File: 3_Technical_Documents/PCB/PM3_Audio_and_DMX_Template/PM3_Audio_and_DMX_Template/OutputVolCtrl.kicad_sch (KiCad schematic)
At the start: 1 part

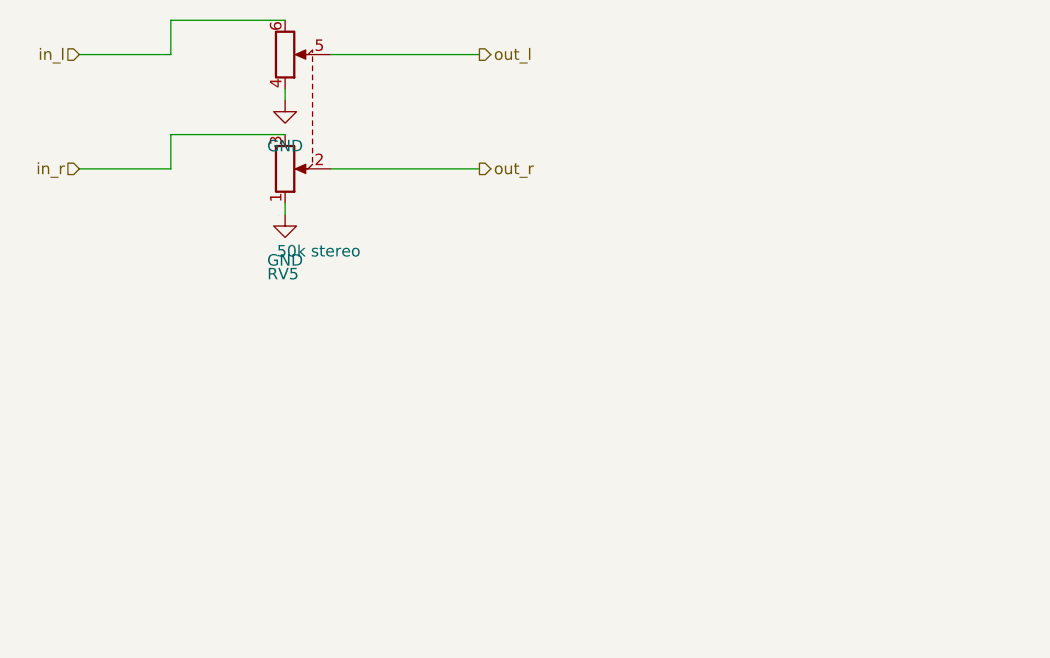
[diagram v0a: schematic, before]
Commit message: new push
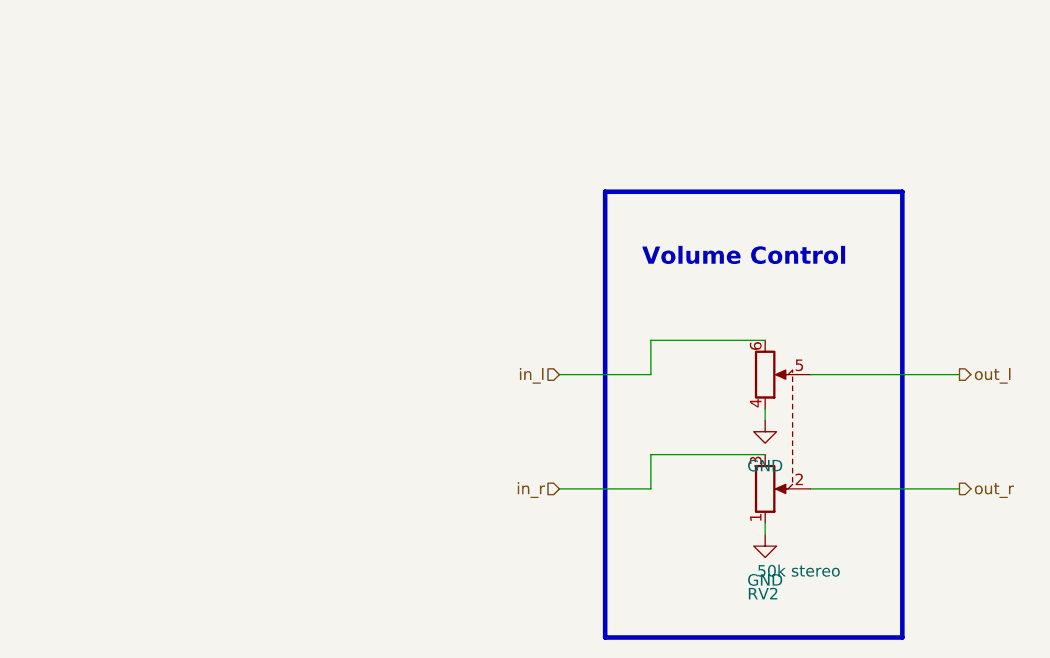
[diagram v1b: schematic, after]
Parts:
- renumbered RV5 to RV2
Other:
- note added: "Volume Control"
- moved on the sheet: RV2
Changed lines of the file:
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@@
 	(generator_version "9.0")
 	(paper "A4")
-	(wire
-		(pts
-			(xy 148.59 88.9) (xy 158.75 88.9)
-		)
-		(stroke
-			(width 0)
-			(type default)
-		)
-	)
-	(wire
-		(pts
-			(xy 158.75 85.09) (xy 171.45 85.09)
-		)
-		(stroke
-			(width 0)
-			(type default)
-		)
-	)
-	(wire
-		(pts
-			(xy 158.75 101.6) (xy 158.75 97.79)
-		)
-		(stroke
-			(width 0)
-			(type default)
-		)
-	)
-	(wire
-		(pts
-			(xy 171.45 105.41) (xy 171.45 106.68)
-		)
-		(stroke
-			(width 0)
-			(type default)
-		)
-	)
-	(wire
-		(pts
-			(xy 158.75 97.79) (xy 171.45 97.79)
-		)
-		(stroke
-			(width 0)
-			(type default)
-		)
-	)
-	(wire
-		(pts
-			(xy 176.53 88.9) (xy 193.04 88.9)
-		)
-		(stroke
-			(width 0)
-			(type default)
-		)
-	)
-	(wire
-		(pts
-			(xy 148.59 101.6) (xy 158.75 101.6)
-		)
-		(stroke
-			(width 0)
-			(type default)
-		)
-	)
-	(wire
-		(pts
-			(xy 176.53 101.6) (xy 193.04 101.6)
-		)
-		(stroke
-			(width 0)
-			(type default)
-		)
-	)
-	(wire
-		(pts
-			(xy 158.75 88.9) (xy 158.75 85.09)
-		)
-		(stroke
-			(width 0)
-			(type default)
-		)
-	)
-	(wire
-		(pts
-			(xy 171.45 92.71) (xy 171.45 93.98)
+	(rectangle
+		(start 207.01 104.14)
+		(end 240.03 153.67)
+		(stroke
+			(width 0.508)
+			(type solid)
+			(color 255 0 0 1)
+		)
+		(fill
+			(type none)
+		)
+	)
+	(text "Volume Control"
+		(exclude_from_sim no)
+		(at 222.504 111.506 0)
+		(effects
+			(font
+				(size 1.905 1.905)
+				(thickness 0.508)
+				(bold yes)
+				(color 255 0 0 1)
+			)
+		)
+	)
+	(wire
+		(pts
+			(xy 201.93 124.46) (xy 212.09 124.46)
+		)
+		(stroke
+			(width 0)
+			(type default)
+		)
+	)
+	(wire
+		(pts
+			(xy 212.09 120.65) (xy 224.79 120.65)
+		)
+		(stroke
+			(width 0)
+			(type default)
+		)
+	)
+	(wire
+		(pts
+			(xy 212.09 137.16) (xy 212.09 133.35)
+		)
+		(stroke
+			(width 0)
+			(type default)
+		)
+	)
+	(wire
+		(pts
+			(xy 224.79 140.97) (xy 224.79 142.24)
+		)
+		(stroke
+			(width 0)
+			(type default)
+		)
+	)
+	(wire
+		(pts
+			(xy 212.09 133.35) (xy 224.79 133.35)
+		)
+		(stroke
+			(width 0)
+			(type default)
+		)
+	)
+	(wire
+		(pts
+			(xy 229.87 124.46) (xy 246.38 124.46)
+		)
+		(stroke
+			(width 0)
+			(type default)
+		)
+	)
+	(wire
+		(pts
+			(xy 201.93 137.16) (xy 212.09 137.16)
+		)
+		(stroke
+			(width 0)
+			(type default)
+		)
+	)
+	(wire
+		(pts
+			(xy 229.87 137.16) (xy 246.38 137.16)
+		)
+		(stroke
+			(width 0)
+			(type default)
+		)
+	)
+	(wire
+		(pts
+			(xy 212.09 124.46) (xy 212.09 120.65)
+		)
+		(stroke
+			(width 0)
+			(type default)
+		)
+	)
+	(wire
+		(pts
+			(xy 224.79 128.27) (xy 224.79 129.54)
 		)
 		(stroke
@@
 	(hierarchical_label "out_r"
 		(shape output)
-		(at 193.04 101.6 0)
+		(at 246.38 137.16 0)
 		(effects
 			(font
@@
 	(hierarchical_label "out_l"
 		(shape output)
-		(at 193.04 88.9 0)
+		(at 246.38 124.46 0)
 		(effects
 			(font
@@
 	(hierarchical_label "in_l"
 		(shape input)
-		(at 148.59 88.9 180)
+		(at 201.93 124.46 180)
 		(effects
 			(font
@@
 	(hierarchical_label "in_r"
 		(shape input)
-		(at 148.59 101.6 180)
+		(at 201.93 137.16 180)
 		(effects
 			(font
@@
 	(symbol
 		(lib_id "power:GND")
-		(at 171.45 106.68 0)
+		(at 224.79 142.24 0)
 		(unit 1)
 		(exclude_from_sim no)
@@
 		(dnp no)
 		(fields_autoplaced yes)
-		(property "Reference" "#PWR030"
-			(at 171.45 113.03 0)
+		(property "Reference" "#PWR038"
+			(at 224.79 148.59 0)
 			(effects
 				(font
@@
 		)
 		(property "Value" "GND"
-			(at 171.45 111.76 0)
+			(at 224.79 147.32 0)
 			(effects
 				(font
@@
 		)
 		(property "Footprint" ""
-			(at 171.45 106.68 0)
+			(at 224.79 142.24 0)
 			(effects
 				(font
@@
 		)
 		(property "Datasheet" ""
-			(at 171.45 106.68 0)
+			(at 224.79 142.24 0)
 			(effects
 				(font
@@
 		)
 		(property "Description" "Power symbol creates a global label with name \"GND\" , ground"
-			(at 171.45 106.68 0)
+			(at 224.79 142.24 0)
 			(effects
 				(font
@@
 			(project "PM3_Audio_and_DMX"
 				(path "/1f276d59-ad9b-4e70-a842-f3b7e562eb9b/2329d9ea-d5d7-4913-84c5-e85a54af032e/396386cb-b8e3-448a-9ee1-2966fe4ed21e"
-					(reference "#PWR030")
+					(reference "#PWR038")
 					(unit 1)
 				)
@@
 	(symbol
 		(lib_id "power:GND")
-		(at 171.45 93.98 0)
+		(at 224.79 129.54 0)
 		(unit 1)
 		(exclude_from_sim no)
@@
 		(dnp no)
 		(fields_autoplaced yes)
-		(property "Reference" "#PWR031"
-			(at 171.45 100.33 0)
+		(property "Reference" "#PWR037"
+			(at 224.79 135.89 0)
 			(effects
 				(font
@@
 		)
 		(property "Value" "GND"
-			(at 171.45 99.06 0)
+			(at 224.79 134.62 0)
 			(effects
 				(font
@@
 		)
 		(property "Footprint" ""
-			(at 171.45 93.98 0)
+			(at 224.79 129.54 0)
 			(effects
 				(font
@@
 		)
 		(property "Datasheet" ""
-			(at 171.45 93.98 0)
+			(at 224.79 129.54 0)
 			(effects
 				(font
@@
 		)
 		(property "Description" "Power symbol creates a global label with name \"GND\" , ground"
-			(at 171.45 93.98 0)
+			(at 224.79 129.54 0)
 			(effects
 				(font
@@
 			(project "PM3_Audio_and_DMX"
 				(path "/1f276d59-ad9b-4e70-a842-f3b7e562eb9b/2329d9ea-d5d7-4913-84c5-e85a54af032e/396386cb-b8e3-448a-9ee1-2966fe4ed21e"
-					(reference "#PWR031")
+					(reference "#PWR037")
 					(unit 1)
 				)
@@
 	(symbol
 		(lib_id "Device:R_Potentiometer_Dual")
-		(at 173.99 95.25 270)
+		(at 227.33 130.81 270)
 		(mirror x)
 		(unit 1)
@@
 		(on_board yes)
 		(dnp no)
-		(property "Reference" "RV5"
-			(at 172.974 113.284 90)
+		(property "Reference" "RV2"
+			(at 226.314 148.844 90)
 			(effects
 				(font
@@
 		)
 		(property "Value" "50k stereo"
-			(at 179.832 110.744 90)
+			(at 233.172 146.304 90)
 			(effects
 				(font
@@
 		)
 		(property "Footprint" "Potentiometer_THT:Potentiometer_Bourns_PTV112-4_Dual_Vertical"
-			(at 172.085 88.9 0)
+			(at 225.425 124.46 0)
 			(effects
 				(font
@@
 		)
 		(property "Datasheet" "~"
-			(at 172.085 88.9 0)
+			(at 225.425 124.46 0)
 			(effects
 				(font
@@
 		)
 		(property "Description" "Dual potentiometer,  PTV112-4420A-A503"
-			(at 173.99 95.25 0)
+			(at 227.33 130.81 0)
 			(effects
 				(font
@@
 		)
 		(property "MPN" ""
-			(at 173.99 95.25 90)
+			(at 227.33 130.81 90)
 			(effects
 				(font
@@
 		)
 		(property "Manufacturer" ""
-			(at 173.99 95.25 90)
+			(at 227.33 130.81 90)
 			(effects
 				(font
@@
 			(project "PM3_Audio_and_DMX"
 				(path "/1f276d59-ad9b-4e70-a842-f3b7e562eb9b/2329d9ea-d5d7-4913-84c5-e85a54af032e/396386cb-b8e3-448a-9ee1-2966fe4ed21e"
-					(reference "RV5")
+					(reference "RV2")
 					(unit 1)
 				)
